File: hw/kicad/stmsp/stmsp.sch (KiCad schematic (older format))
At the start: 1 part, among them P2 CONN_02X07

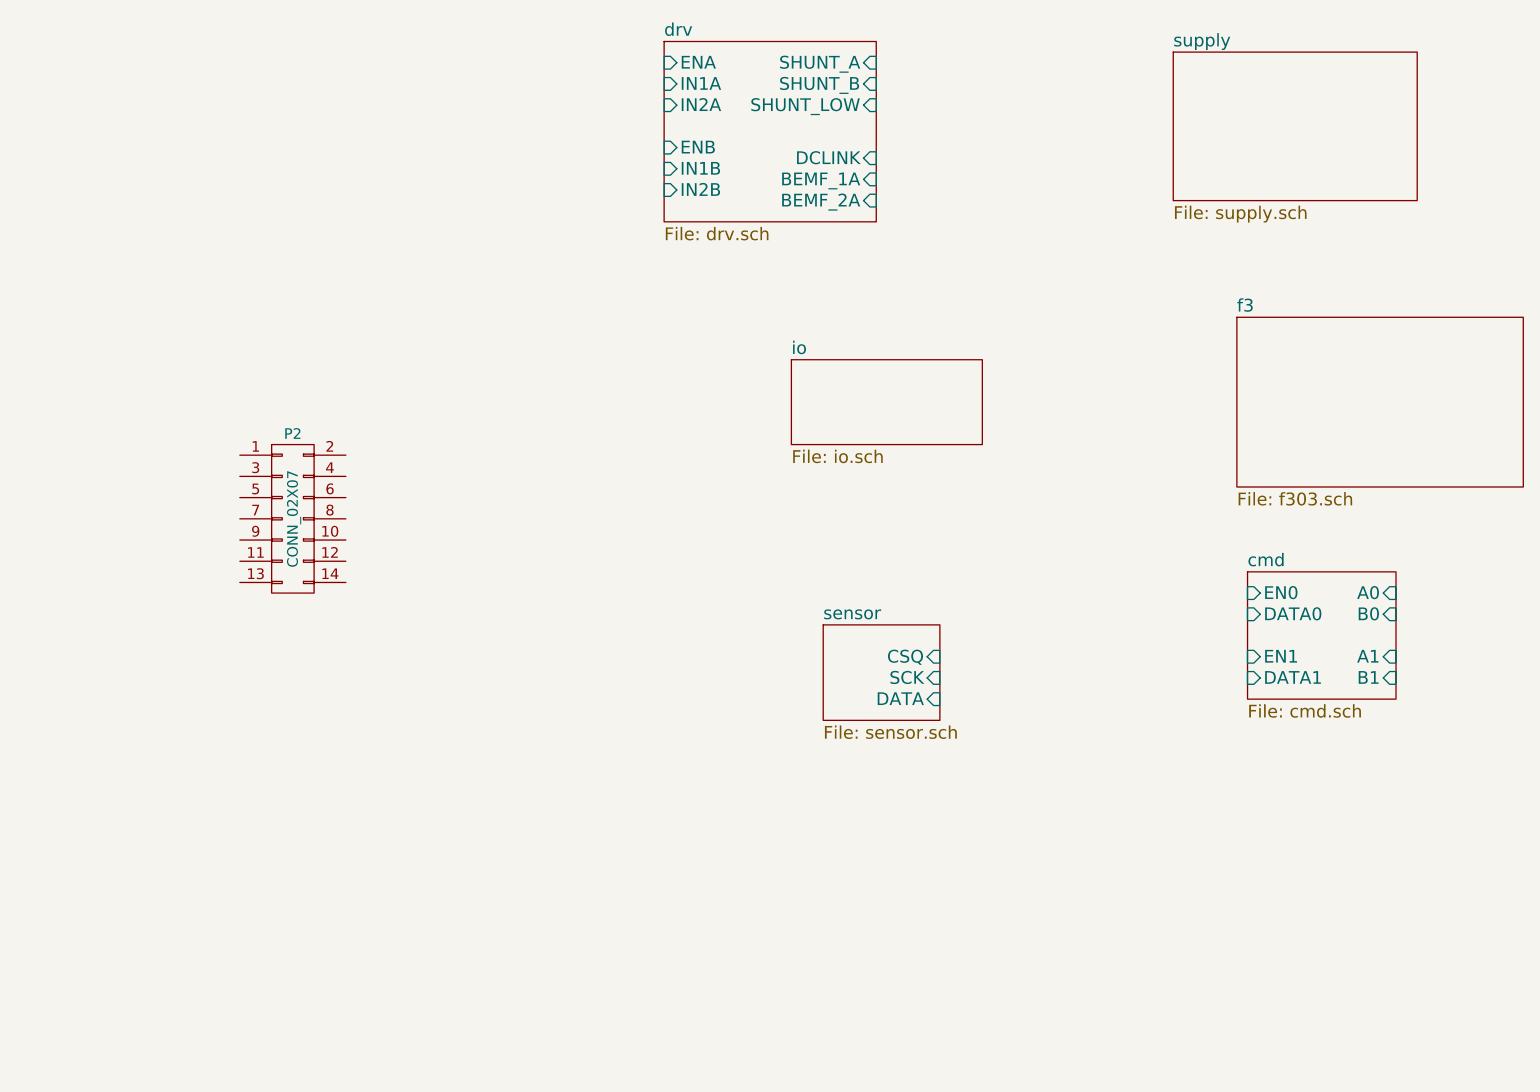
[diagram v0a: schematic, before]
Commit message: stmsp
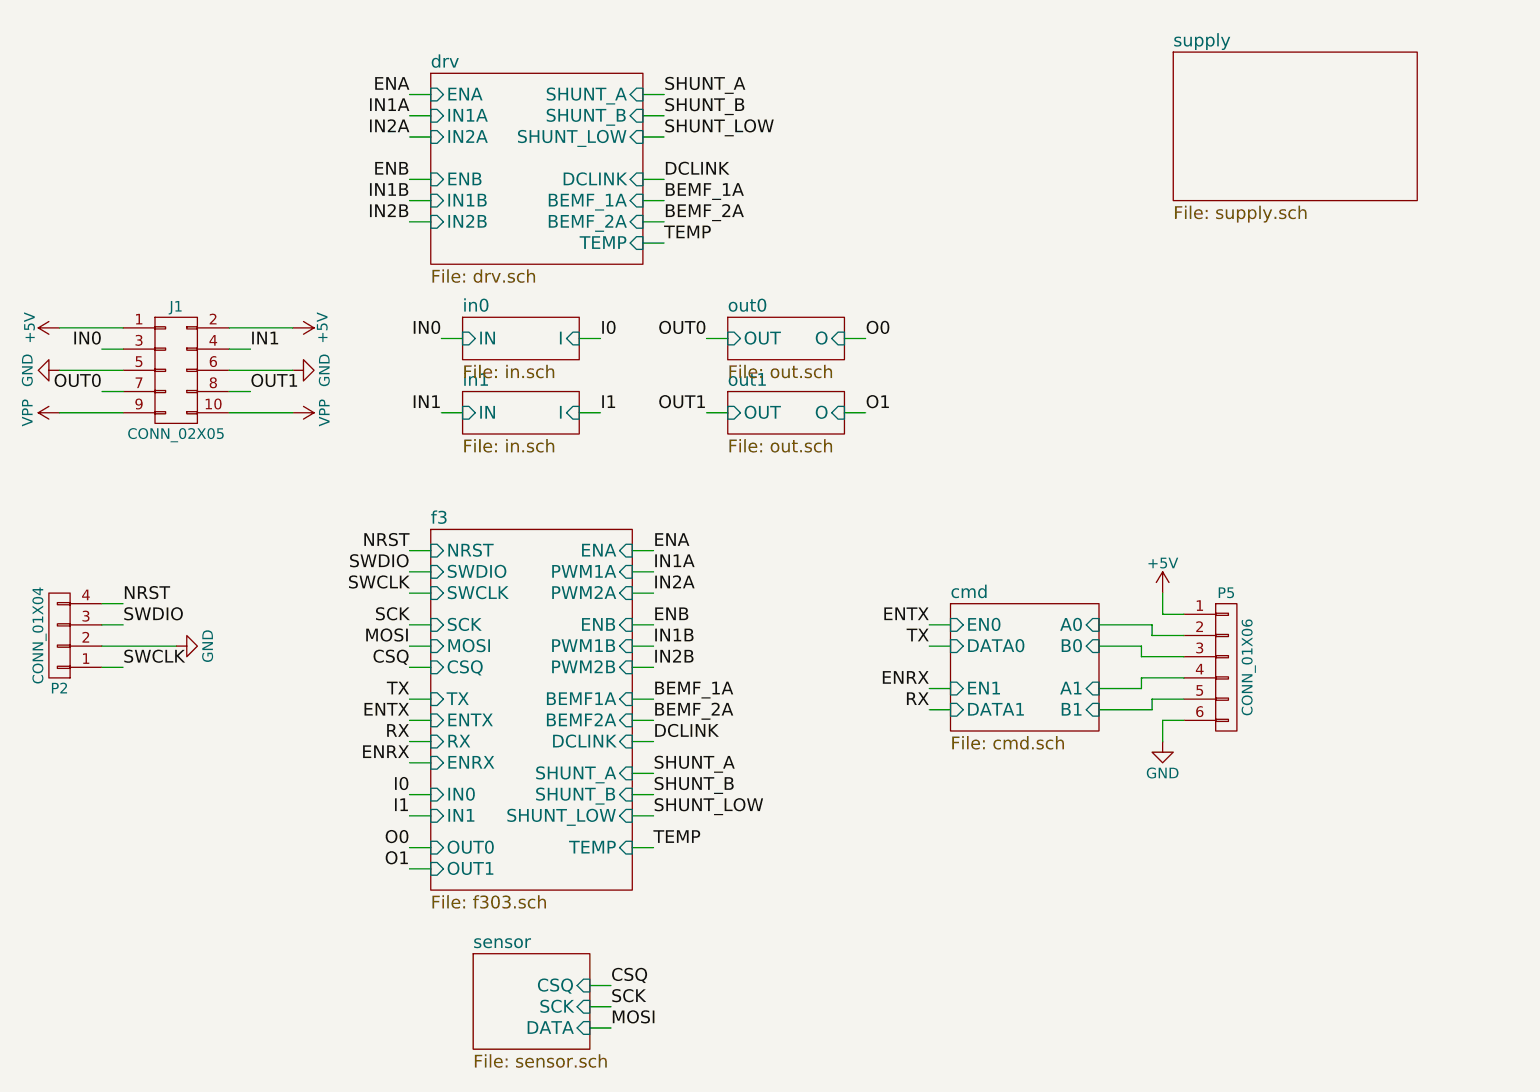
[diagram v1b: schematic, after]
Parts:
- removed P2: CONN_02X07, Pin_Headers:Pin_Header_Straight_2x07, symbol CONN_02X07
- added J1: CONN_02X05, Pin_Headers:Pin_Header_Straight_2x05, symbol CONN_02X05
- added P2: CONN_01X04, Pin_Headers:Pin_Header_Straight_1x04, symbol CONN_01X04
- added P5: CONN_01X06, Pin_Headers:Pin_Header_Straight_1x06, symbol CONN_01X06
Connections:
- net cmd/A0: now also P5.2 (P2)
- net cmd/A1: now also P5.4 (P4)
- net cmd/B0: now also P5.3 (P3)
- net cmd/B1: now also P5.5 (P5)
- new net +5V: J1.1 (P1), J1.2 (P2), P5.1 (P1)
- new net GND: J1.5 (P5), J1.6 (P6), P2.2 (P2), P5.6 (P6)
- new net IN0: J1.3 (P3)
- new net IN1: J1.4 (P4)
- new net NRST: P2.4 (P4)
- new net OUT0: J1.7 (P7)
- new net OUT1: J1.8 (P8)
- new net SWCLK: P2.1 (P1)
- new net SWDIO: P2.3 (P3)
- new net VPP: J1.10 (P10), J1.9 (P9)

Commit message: stmsp
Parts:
- J1: footprint Pin_Headers:Pin_Header_Straight_2x05 -> stmbl:Pin_Header_Straight_2x05
- P2: footprint Pin_Headers:Pin_Header_Straight_1x04 -> stmbl:Pin_Header_Straight_1x04
- P5: footprint Pin_Headers:Pin_Header_Straight_1x06 -> stmbl:Pin_Header_Straight_1x06
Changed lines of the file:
@@
 F 0 "P5" H 8200 5900 50  0000 C CNN
 F 1 "CONN_01X06" V 8300 5550 50  0000 C CNN
-F 2 "Pin_Headers:Pin_Header_Straight_1x06" H 8200 5550 50  0001 C CNN
+F 2 "stmbl:Pin_Header_Straight_1x06" H 8200 5550 50  0001 C CNN
 F 3 "" H 8200 5550 50  0000 C CNN
 	1    8200 5550
@@
 F 0 "J1" H 3250 4450 50  0000 C CNN
 F 1 "CONN_02X05" H 3250 3850 50  0000 C CNN
-F 2 "Pin_Headers:Pin_Header_Straight_2x05" H 3250 2950 50  0001 C CNN
+F 2 "stmbl:Pin_Header_Straight_2x05" H 3250 2950 50  0001 C CNN
 F 3 "" H 3250 2950 50  0001 C CNN
 	1    3250 4150
@@
 F 0 "P2" H 2700 5650 50  0000 C CNN
 F 1 "CONN_01X04" V 2800 5400 50  0000 C CNN
-F 2 "Pin_Headers:Pin_Header_Straight_1x04" H 2700 5400 50  0001 C CNN
+F 2 "stmbl:Pin_Header_Straight_1x04" H 2700 5400 50  0001 C CNN
 F 3 "" H 2700 5400 50  0000 C CNN
 	1    2700 5400
